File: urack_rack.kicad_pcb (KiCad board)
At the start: 2 copper layers, 210 x 154.5 mm, 20 parts, among them J1 Conn_01x40, J10 105450-0101, J11 105450-0101, J12 105450-0101, J2 Conn_01x40, J3 Conn_01x40, J4 Conn_01x40, J5 Conn_02x40_Odd_Even, J6 Conn_02x40_Odd_Even, J7 Conn_02x40_Odd_Even, J8 Conn_02x40_Odd_Even, J9 105450-0101

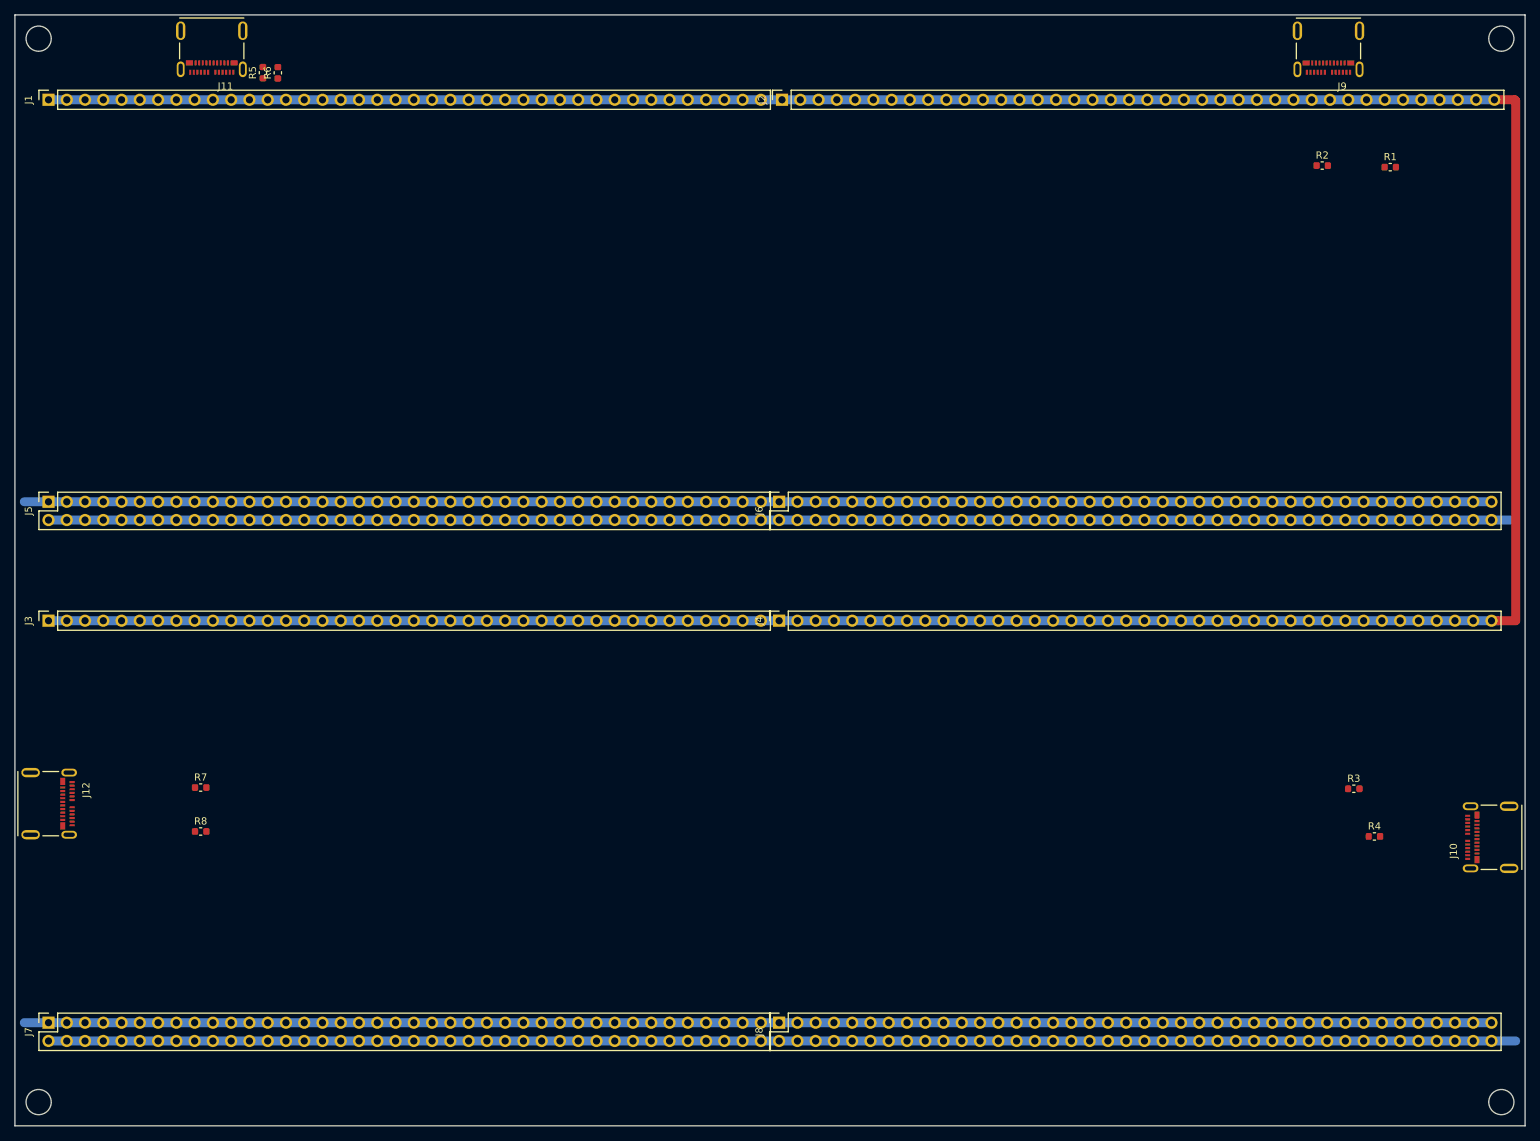
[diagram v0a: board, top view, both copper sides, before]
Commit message: Update PCB
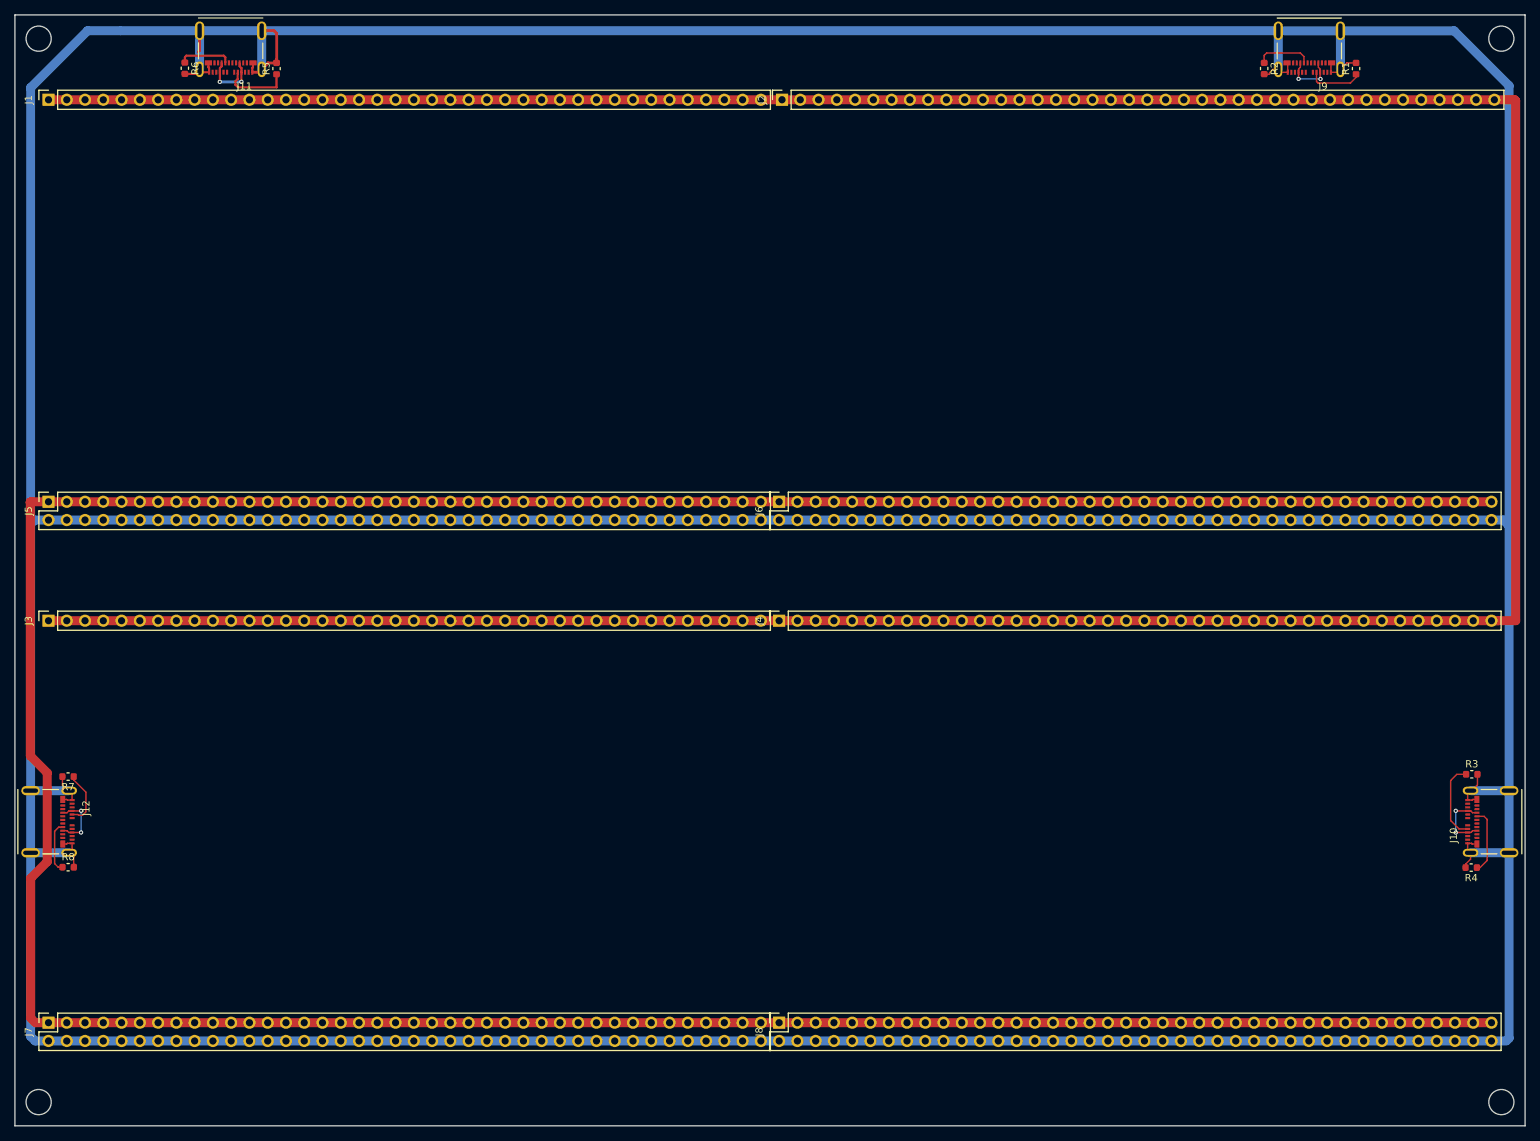
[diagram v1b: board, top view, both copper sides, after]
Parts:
- moved R8 19.1 mm to (27.4, 138.5)
- moved R7 18.5 mm to (27.4, 125.9), turned to 180 degrees
- moved R3 16.5 mm to (222.6, 125.6)
- moved R2 15.7 mm to (193.7, 27.5), turned to 270 degrees
- moved R1 14.5 mm to (206.5, 27.5), turned to 90 degrees
- moved R4 14.1 mm to (222.5, 138.6), turned to 180 degrees
- moved R6 12.9 mm to (43.6, 27.4), turned to 270 degrees
- moved J9 2.66 mm to (200.0, 24.2)
- moved J11 2.63 mm to (50.0, 24.2)
- moved J12 2.51 mm to (24.2, 132.2)
- moved J10 2.17 mm to (225.8, 132.2)
- moved R5 1.97 mm to (56.4, 27.5)
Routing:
- net GND: track 408.1 -> 982.9 mm
- net -9V: track 408.1 -> 480.3 mm
- net +5V: track 0.00 -> 33.7 mm, vias 0 -> 8
- net Net-(J10-PadA5): track 0.00 -> 10.9 mm
- net Net-(J11-PadA5): track 0.00 -> 9.58 mm
- net Net-(J10-PadB5): track 0.00 -> 9.15 mm
- net Net-(J9-PadB5): track 0.00 -> 7.80 mm
- net Net-(J12-PadA5): track 0.00 -> 7.75 mm
- net Net-(J9-PadA5): track 0.00 -> 7.63 mm
- net Net-(J11-PadB5): track 0.00 -> 7.32 mm
- net Net-(J12-PadB5): track 0.00 -> 7.17 mm
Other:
- net class Default: clearance 0.6 -> 0.15; trace_width 1.25 -> 0.2; via_dia 1 -> 0.6; via_drill 0.6 -> 0.3
- rule trace_clearance: 0.6 -> 0.15
